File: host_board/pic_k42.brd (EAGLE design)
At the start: 54.6 x 77.5 mm, 53 parts, among them IC1 PIC18F57K42-E_PT, IC2 REF3440IDBVR, IC3 MAX232, IC4 ILAMP, K1 G6K-2P, Q1 ASF1, X1 RX-2, X2 TX-2, X3 RESETJMP, X5 PORTA, X6 PORTD, X7 PORTB

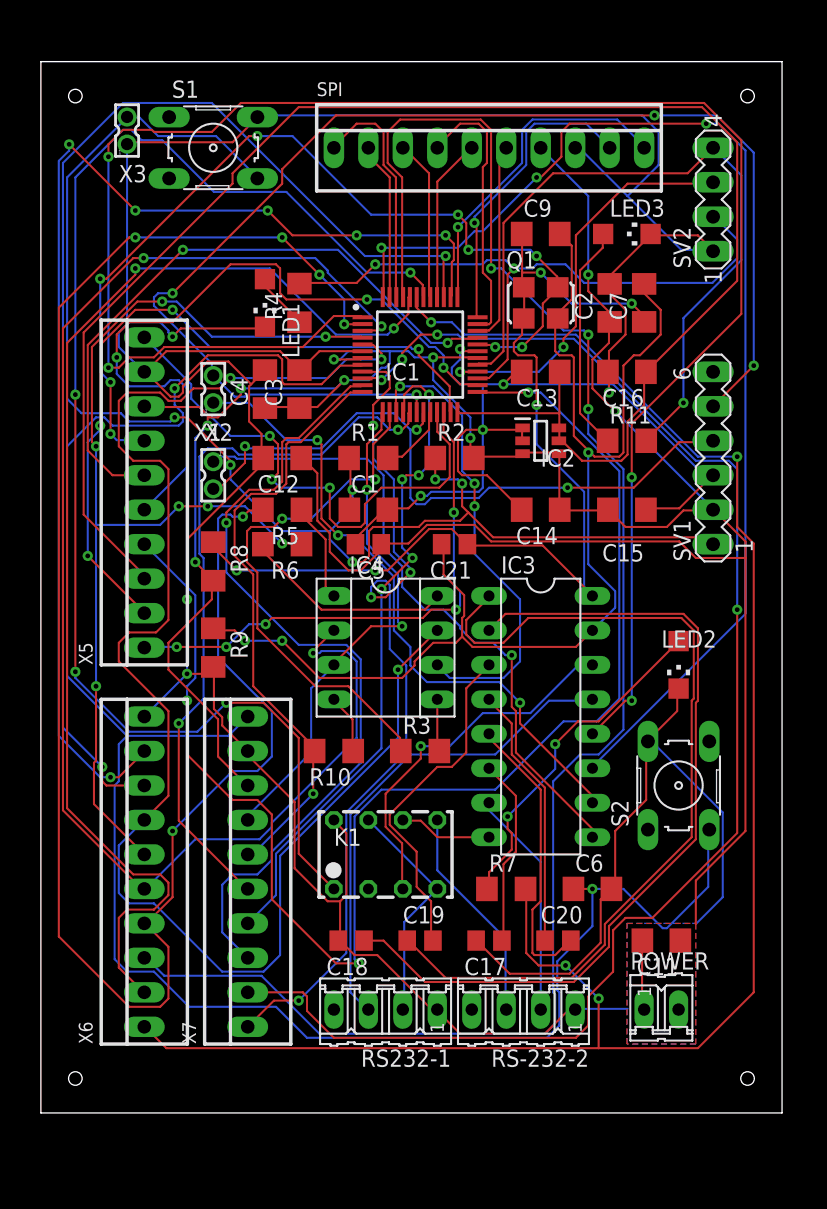
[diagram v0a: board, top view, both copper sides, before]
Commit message: new board
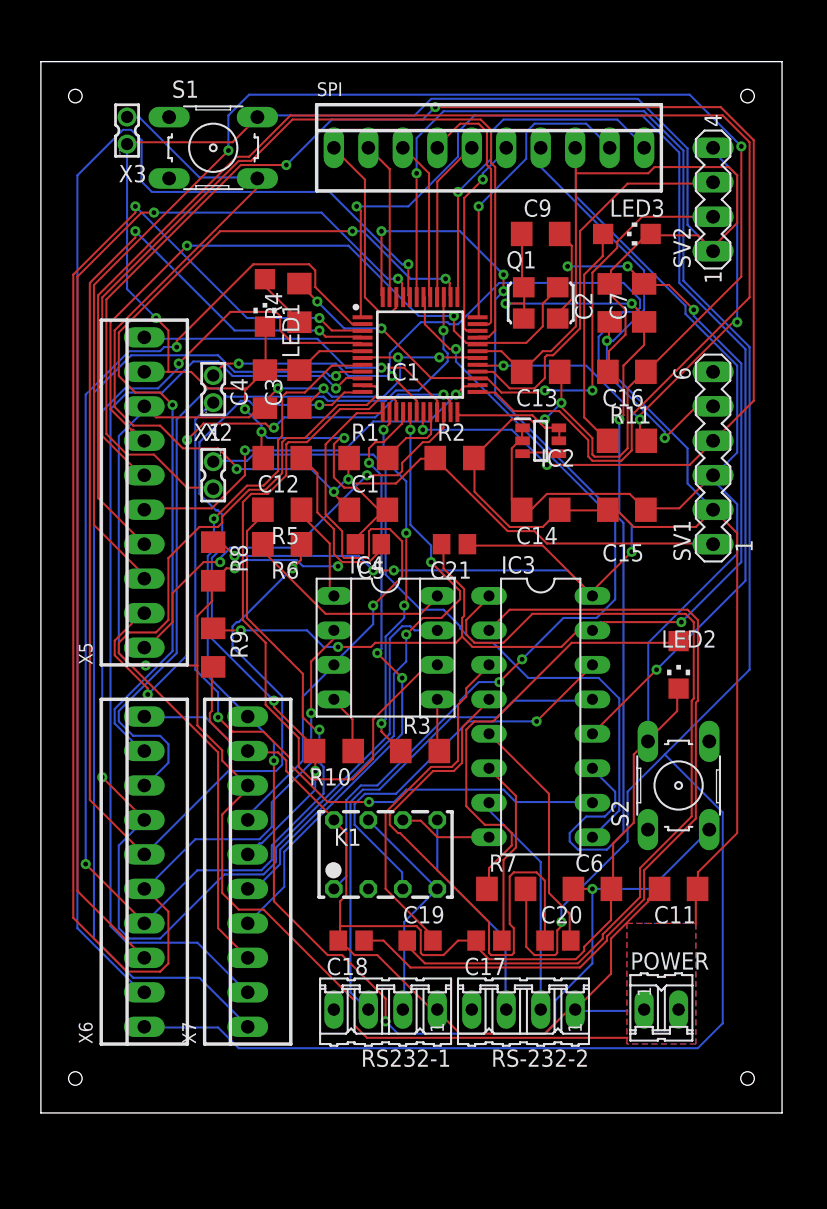
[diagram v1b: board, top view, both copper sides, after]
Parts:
- moved C11 4.02 mm to (71.1, 11.4)
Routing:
- net N$6: track 49.6 -> 122.0 mm, vias 3 -> 4
- net N$18: track 134.5 -> 86.6 mm, vias 4 -> 2
- net N$45: track 128.1 -> 81.3 mm, vias 3 -> 2
- net N$43: track 142.7 -> 98.0 mm, vias 2 -> 4
- net N$52: track 131.3 -> 172.9 mm, vias 4 -> 2
- net N$28: track 101.8 -> 61.4 mm, vias 4 -> 3
- net N$7: track 96.0 -> 58.8 mm, vias 4 -> 3
- net N$54: track 107.6 -> 71.4 mm, vias 4 -> 1
- net VDD: track 212.7 -> 245.1 mm, vias 9 -> 8
- net N$51: track 87.8 -> 59.6 mm, vias 2 -> 1
- net N$35: track 53.2 -> 29.4 mm, vias 3 -> 2
- net N$48: track 78.4 -> 101.8 mm, vias 7 -> 3
- net N$46: track 131.5 -> 109.7 mm, vias 6 -> 3
- net N$11: track 19.5 -> 40.9 mm
- net N$50: track 87.7 -> 66.5 mm, vias 6 -> 3
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
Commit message: update
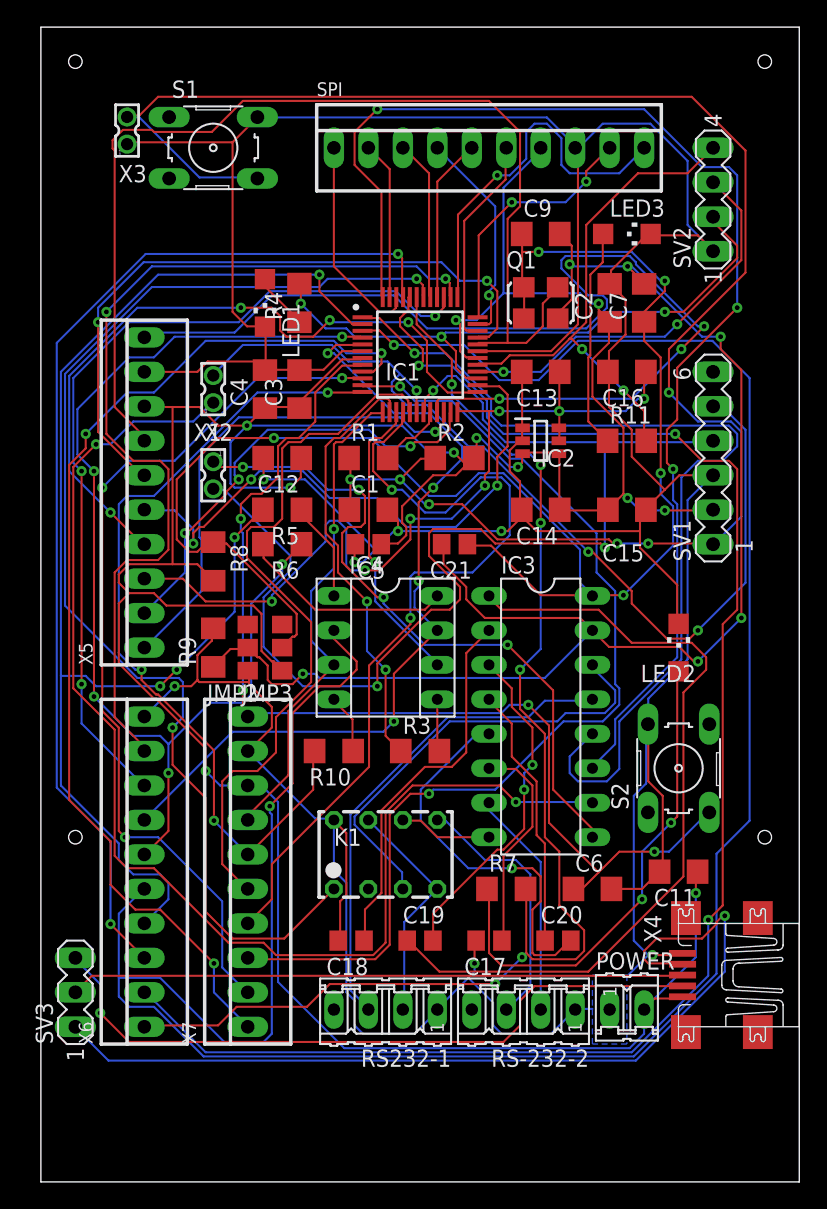
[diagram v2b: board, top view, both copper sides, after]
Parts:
- added JMP2, JMP3: 0R-JUMPA, jump-0r-smd:A0R-JMP
- added SV3: USBH, con-lstb:MA03-1
- added X4: MINI-USB-UX60A-MB-5ST, con-hirose:UX60A-MB-5ST
- moved POWER 2.54 mm to (67.3, 2.54)
- moved C11 1.27 mm to (71.1, 12.7)
- moved LED2 1.27 mm to (71.1, 29.2), turned to 0 degrees
- moved S2 1.27 mm to (71.1, 20.3)
- turned R9 to 90 degrees
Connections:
- new net N$67: SV3.1, X4.4
- new net N$68: SV3.2, X4.3
- new net N$69: SV3.3, X4.2
- net GND: now also JMP2.2
- net VCC: now also JMP3.2
- net VDD: now also JMP3.1, X4.1
- net VSS: now also JMP2.1, X4.5
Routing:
- net N$52: track 172.9 -> 95.2 mm, vias 2 -> 6
- net N$67: track 0.00 -> 66.4 mm, vias 0 -> 1
- net N$47: track 117.7 -> 181.9 mm, vias 3 -> 2
- net N$8: track 126.8 -> 62.9 mm, vias 4 -> 7
- net N$36: track 114.9 -> 52.6 mm, vias 0 -> 4
- net N$39: track 24.4 -> 78.2 mm, vias 1 -> 3
- net N$69: track 0.00 -> 51.4 mm, vias 0 -> 1
- net N$68: track 0.00 -> 45.3 mm
- net N$1: track 86.8 -> 131.2 mm, vias 3 -> 6
- net N$49: track 102.3 -> 60.7 mm, vias 2 -> 4
- net N$22: track 55.7 -> 91.8 mm
- net N$9: track 62.3 -> 27.9 mm
- net N$6: track 122.0 -> 87.6 mm, vias 4 -> 3
- net VCC: track 81.9 -> 115.8 mm, vias 7 -> 5
- net N$60: track 53.7 -> 21.9 mm, vias 0 -> 1
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- removed copper zone on layer 1, net VDD
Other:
- board size 54.6 x 77.5 mm -> 55.9 x 85.1 mm
- board text added: "1.4"
- board text removed: "1.3"

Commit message: update
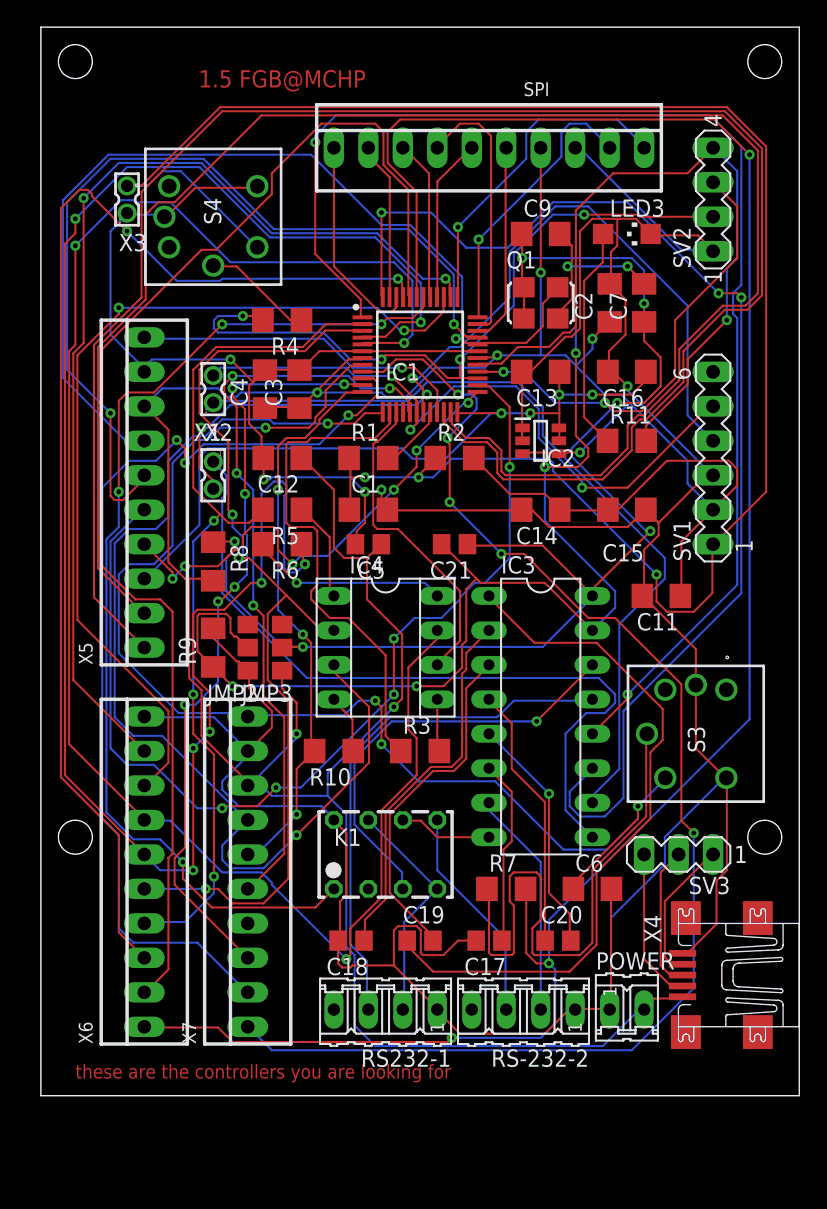
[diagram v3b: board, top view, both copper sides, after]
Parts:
- removed LED1: RUN, led:CHIPLED_1206
- removed LED2: MODE, led:CHIPLED_1206
- removed S1: RESETSW, switch-omron:B3F-10XX
- removed S2: MODESW, switch-omron:B3F-10XX
- added S3: MODE SW, SamacSys_Parts:B3W-9_1-LED
- added S4: RESET SW, SamacSys_Parts:B3W-9_1-LED
- moved SV3 45.6 mm to (71.1, 14.0), turned to 180 degrees
- moved C11 20.4 mm to (69.8, 33.0)
- moved X3 5.08 mm to (30.5, 62.2)
- moved R4 1.80 mm to (41.9, 53.3), turned to 180 degrees
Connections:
- net N$1: now also S4.4; no longer S1.4
- net N$21: now also S4.5; no longer LED1.A
- net N$43: now also S3.4; no longer S2.3
- net N$64: now also S3.5; no longer LED2.A
- net VSS: now also S3.2, S3.6, S4.2, S4.6; no longer LED1.C, LED2.C, S1.2, S2.2
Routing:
- net N$47: track 181.9 -> 71.7 mm, vias 2 -> 3
- net N$38: track 36.6 -> 131.5 mm, vias 1 -> 0
- net N$37: track 33.4 -> 125.8 mm, vias 3 -> 0
- net N$49: track 60.7 -> 128.2 mm, vias 4 -> 3
- net N$56: track 61.0 -> 0.00 mm, vias 2 -> 0
- net N$67: track 66.4 -> 10.7 mm, vias 1 -> 0
- net N$48: track 81.0 -> 136.3 mm, vias 5 -> 7
- net N$52: track 95.2 -> 149.6 mm, vias 6 -> 3
- net N$39: track 78.2 -> 24.8 mm, vias 3 -> 1
- net N$59: track 36.3 -> 78.4 mm, vias 1 -> 2
- net N$69: track 51.4 -> 11.4 mm, vias 1 -> 0
- net N$68: track 45.3 -> 10.6 mm
- net N$46: track 97.0 -> 64.5 mm, vias 4 -> 3
- net VSS: track 343.6 -> 311.3 mm, vias 7 -> 5
- net N$35: track 42.8 -> 74.3 mm, vias 3 -> 5
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- removed copper zone on layer 16, net VSS
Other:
- board size 55.9 x 85.1 mm -> 55.9 x 78.7 mm
- board text added: "/fred/Downloads/mchp.bmp"
- board text added: "1.5 FGB@MCHP"
- board text added: "these are the controllers you are looking for"
- board text removed: "1.4"
